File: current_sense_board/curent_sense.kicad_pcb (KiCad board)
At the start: 2 copper layers, 50.4 x 63 mm, 19 parts, among them J1 Screw_Terminal_01x01, J10 Conn_01x05_Pin, J2 Screw_Terminal_01x01, J3 Screw_Terminal_01x01, J4 Screw_Terminal_01x01, J7 Screw_Terminal_01x01, J8 Screw_Terminal_01x01, U1 ACS758KCB-150B-PFF-T, U2 ACS758KCB-150B-PFF-T, U8 ACS758KCB-150B-PFF-T

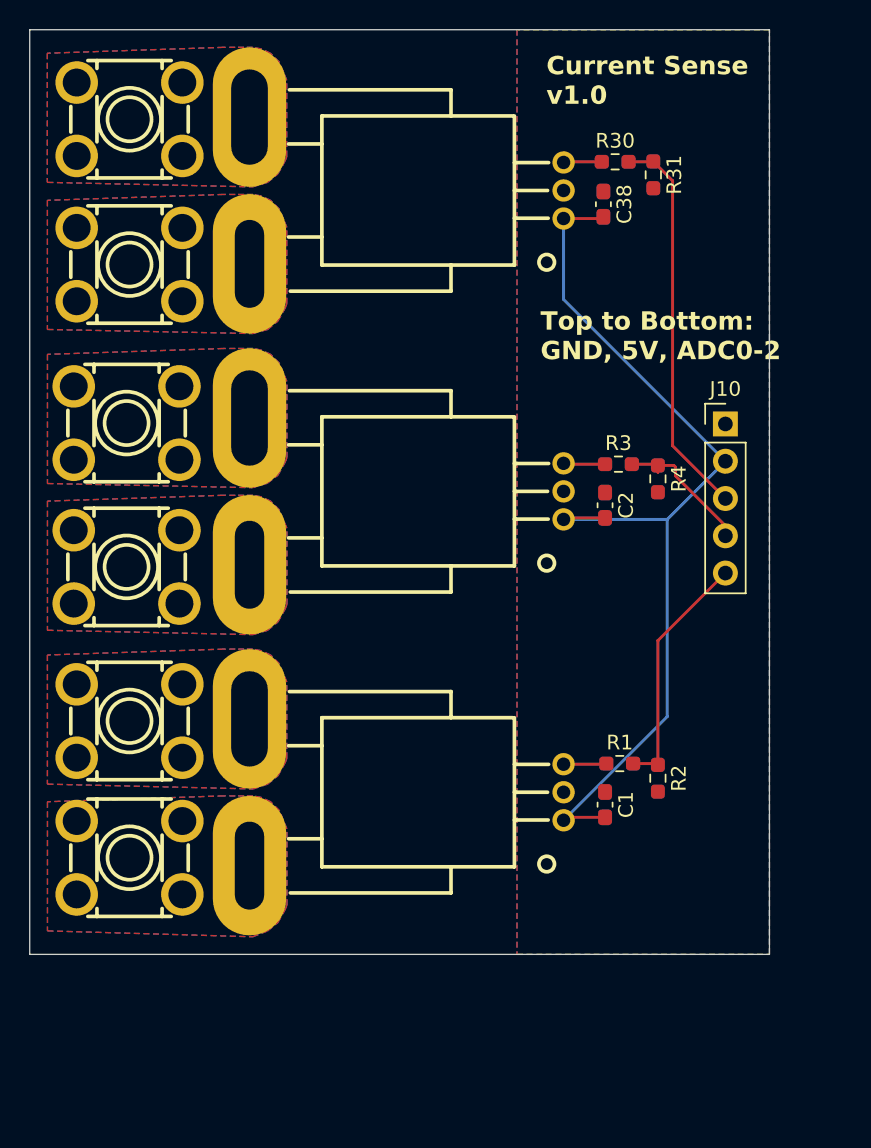
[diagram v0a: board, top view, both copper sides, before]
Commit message: did stuff
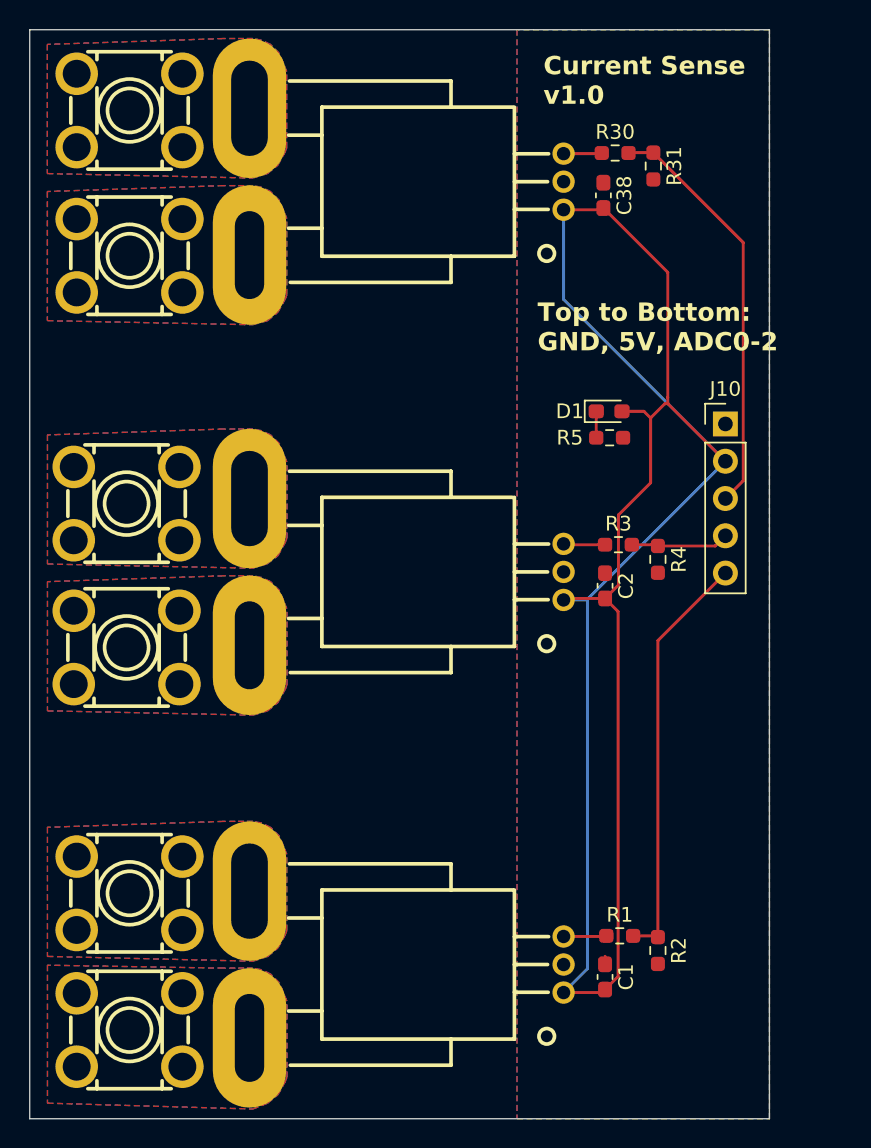
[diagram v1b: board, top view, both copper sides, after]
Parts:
- added D1: LED, LED_SMD:LED_0603_1608Metric_Pad1.05x0.95mm_HandSolder, F.Cu at (82.1, 74.4)
- added R5: 330, Resistor_SMD:R_0603_1608Metric_Pad0.98x0.95mm_HandSolder, F.Cu at (82.1, 76.2)
- moved U1 11.7 mm to (68.3, 112.1)
- moved J1 11.7 mm to (49.4, 116.6)
- moved J2 11.7 mm to (49.4, 107.2)
- moved C1 11.7 mm to (81.8, 112.9)
- moved R1 11.7 mm to (82.8, 110.1)
- moved R2 11.7 mm to (85.4, 111.1)
- moved U2 5.49 mm to (68.3, 85.3)
- moved C2 5.49 mm to (81.8, 86.3)
- moved J3 5.49 mm to (49.2, 90.5)
- moved J4 5.49 mm to (49.2, 80.7)
- moved R3 5.49 mm to (82.7, 83.5)
- moved R4 5.49 mm to (85.4, 84.5)
- moved J7 0.60 mm to (49.4, 63.8)
- moved C38 0.60 mm to (81.7, 59.7)
- moved J8 0.60 mm to (49.4, 53.9)
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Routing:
- net +5V: track 66.0 -> 138.0 mm
- net /ADC2: track 16.7 -> 28.4 mm
- net /ADC1: track 9.80 -> 6.70 mm
- net Net-(D1-K): track 0.00 -> 1.80 mm
- net /ADC0: track 26.7 -> 28.3 mm
- net GND: track 0.00 -> 0.54 mm
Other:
- board size 50.4 x 63 mm -> 50.4 x 74.2 mm
